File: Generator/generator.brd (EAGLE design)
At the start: 100 x 80 mm, 28 parts, among them IC2 317EMP, X1 22-23-2021

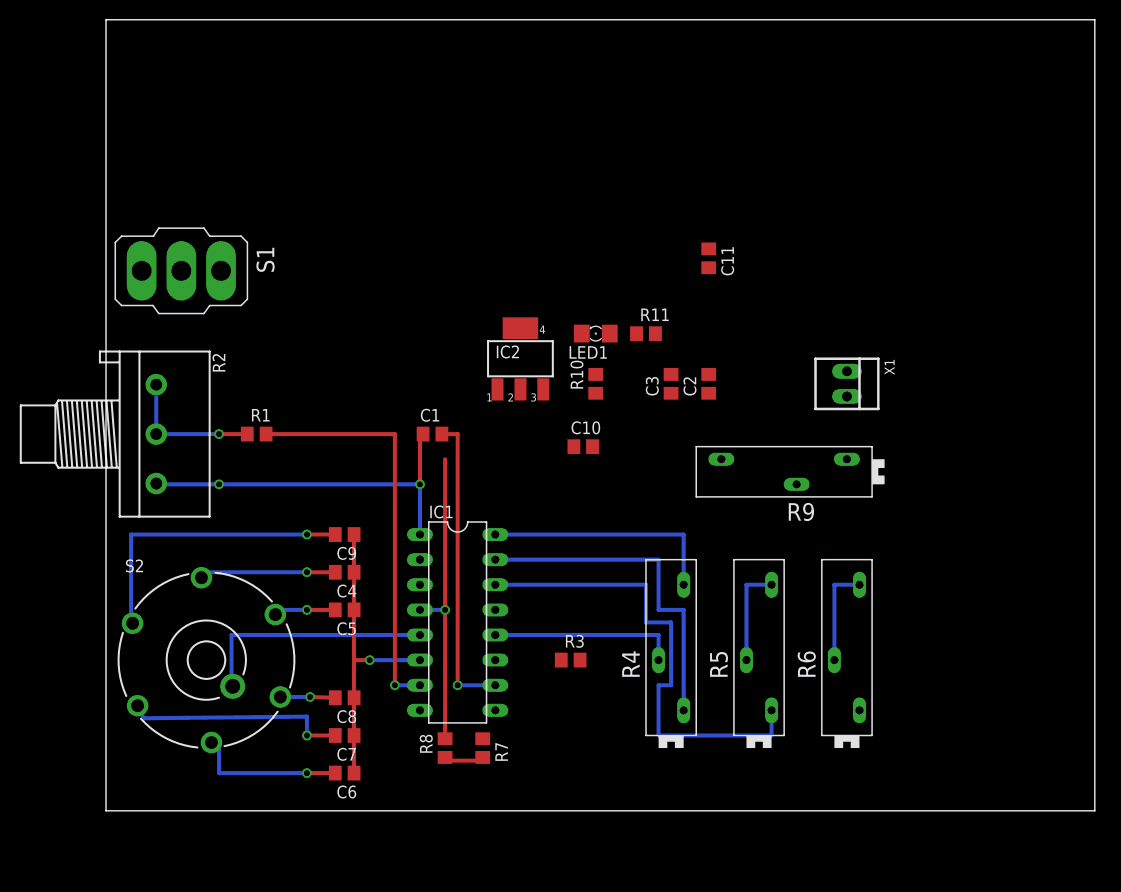
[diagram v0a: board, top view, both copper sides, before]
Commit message: test
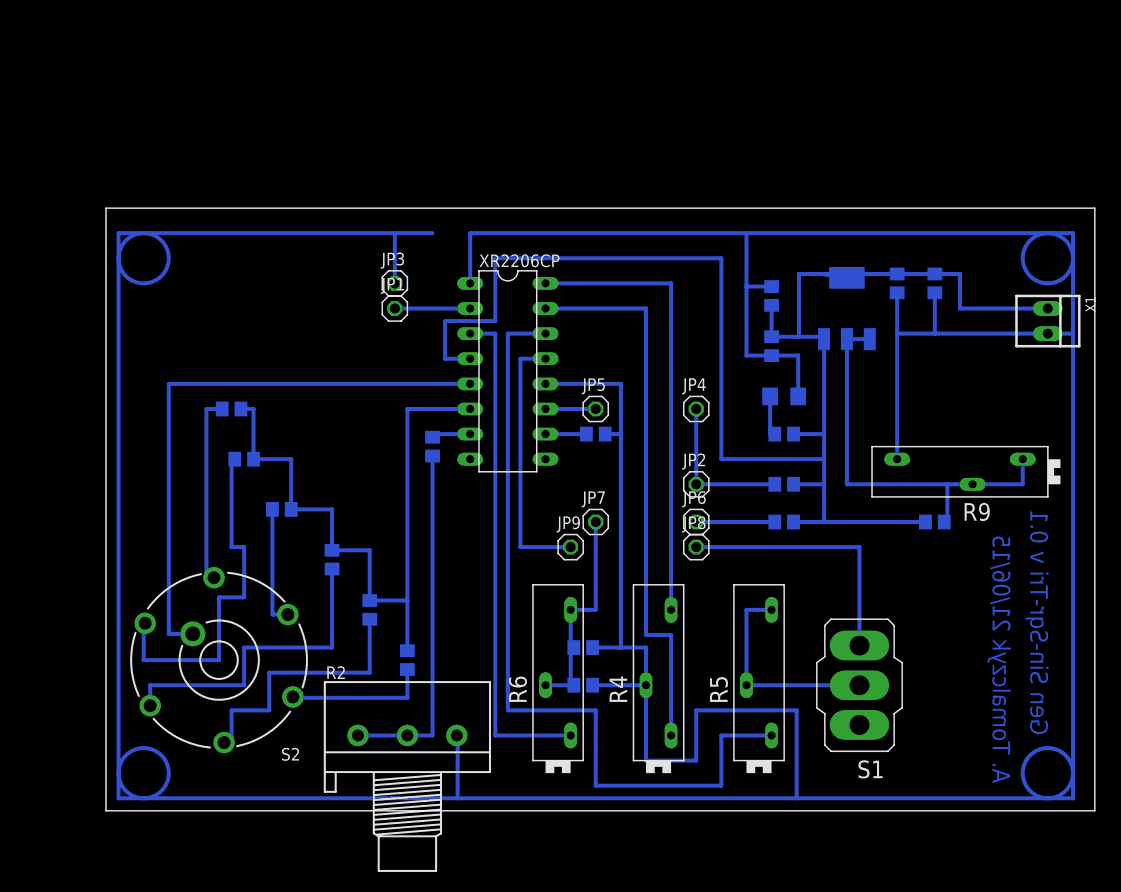
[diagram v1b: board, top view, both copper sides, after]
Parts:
- removed IC1: (no value), exar:DIL16
- added C12: 10uF, rcl:C0805
- added JP1, JP2, JP3, JP4, JP5, JP6, JP7, JP8, JP9: (no value), pinhead:1X01
- added XR2206CP: (no value), exar:DIL16
- moved S1 80.4 mm to (76.2, 12.7), turned to 180 degrees
- moved R8 41.2 mm to (68.6, 29.2), flipped to the bottom, turned to 180 degrees
- moved R2 39.7 mm to (30.5, 7.62), turned to 0 degrees
- moved C10 39.2 mm to (83.8, 53.3), flipped to the bottom, turned to 90 degrees
- moved C6 38.6 mm to (12.7, 40.6), flipped to the bottom, turned to 0 degrees
- moved R10 37.0 mm to (83.8, 29.2), flipped to the bottom, turned to 0 degrees
- moved IC2 33.4 mm to (74.9, 50.8), flipped to the bottom
- moved R6 29.3 mm to (45.7, 14.0)
- moved R3 28.0 mm to (68.6, 33.0), flipped to the bottom, turned to 180 degrees
- moved C8 26.2 mm to (14.0, 35.6), flipped to the bottom, turned to 0 degrees
- moved C7 23.7 mm to (17.8, 30.5), flipped to the bottom, turned to 0 degrees
- moved X1 21.3 mm to (95.2, 49.5)
- moved LED1 20.1 mm to (68.6, 41.9), flipped to the bottom
- moved C11 19.2 mm to (80.0, 53.3), flipped to the bottom
- moved R1 17.8 mm to (33.0, 36.8), flipped to the bottom, turned to 90 degrees
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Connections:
- net C2: now also XR2206CP.6; no longer IC1.6
- net GND: now also C12.2, JP3.1, XR2206CP.1, XR2206CP.12; no longer IC1.1, IC1.12
- net N$10: now also XR2206CP.10; no longer IC1.10
- net N$11: now also C12.1
- net N$12: now also XR2206CP.15; no longer IC1.15
- net N$13: now also XR2206CP.16; no longer IC1.16
- net N$14: now also XR2206CP.14; no longer IC1.14
- net N$15: now also XR2206CP.13; no longer IC1.13
- net N$17: now also XR2206CP.3; no longer IC1.3
- net N$2: now also XR2206CP.5; no longer IC1.5
- net N$7: now also XR2206CP.7; no longer IC1.7
- net SIN_TRI: now also JP1.1, XR2206CP.2; no longer IC1.2
- net SQR: now also JP2.1, XR2206CP.11; no longer IC1.11
- net VCC: now also XR2206CP.4; no longer IC1.4
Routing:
- net GND: track 56.3 -> 470.5 mm, vias 2 -> 0
- net VCC: track 30.8 -> 155.7 mm, vias 1 -> 0
- net N$15: track 0.00 -> 53.1 mm
- net N$17: track 0.00 -> 50.8 mm
- net N$19: track 0.00 -> 41.4 mm
- net N$7: track 41.0 -> 4.13 mm, vias 1 -> 0
- net C2: track 30.8 -> 67.0 mm, vias 1 -> 0
- net N$2: track 24.4 -> 58.2 mm
- net N$14: track 48.3 -> 81.3 mm
- net N$4: track 5.55 -> 35.9 mm, vias 1 -> 0
- net N$10: track 30.8 -> 4.13 mm, vias 1 -> 0
- net N$3: track 6.53 -> 32.2 mm, vias 1 -> 0
- net N$9: track 14.2 -> 35.8 mm, vias 1 -> 0
- net N$13: track 24.1 -> 45.7 mm
- net N$12: track 34.3 -> 55.9 mm
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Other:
- board size 100 x 80 mm -> 100 x 61 mm
- board text added: "A. Tomalczyk 21/06/15"
- board text added: "Gen Sin-Sqr-Tri v 0.1"
